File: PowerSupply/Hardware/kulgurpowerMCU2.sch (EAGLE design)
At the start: 140 parts, among them IC2 TPS77333DGK, IC3 REG1117-5, U1 MPU-6000QFN-24, U2 MPU-6000QFN-24, X1 12Mhz

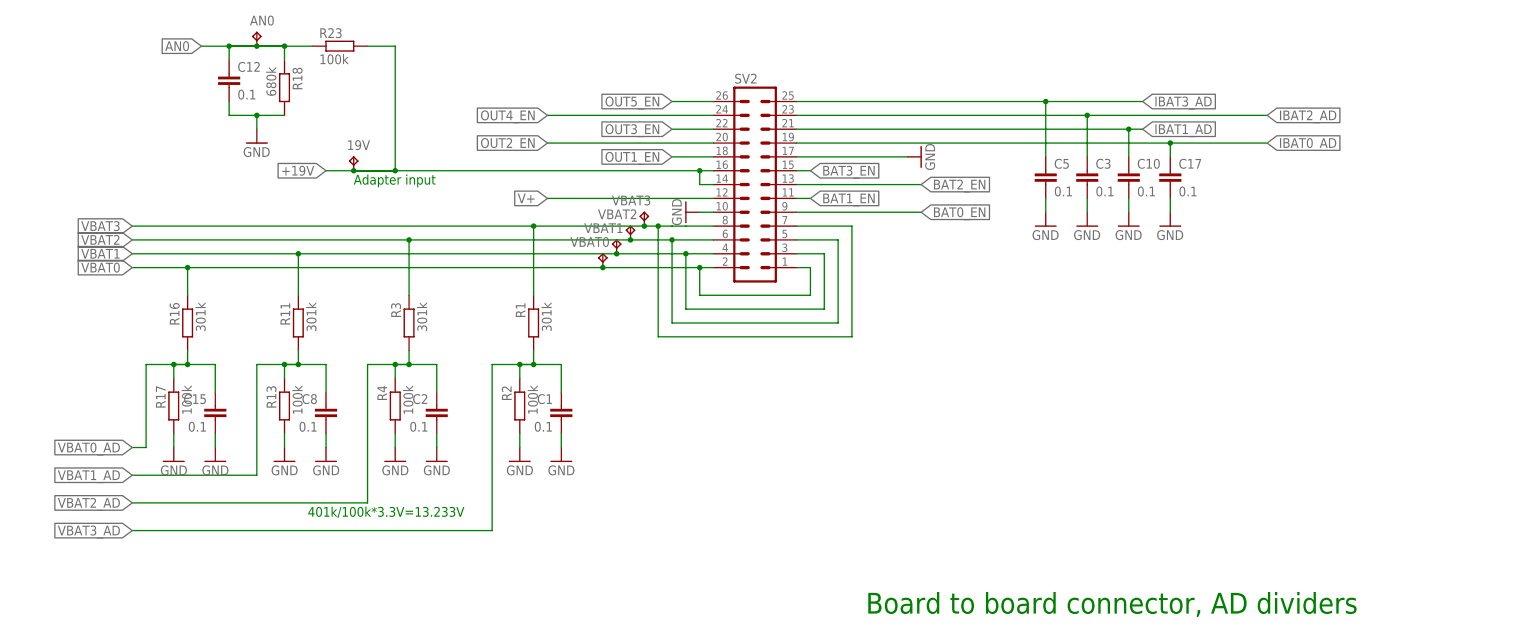
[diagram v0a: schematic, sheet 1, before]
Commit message: lot of work done on schematics
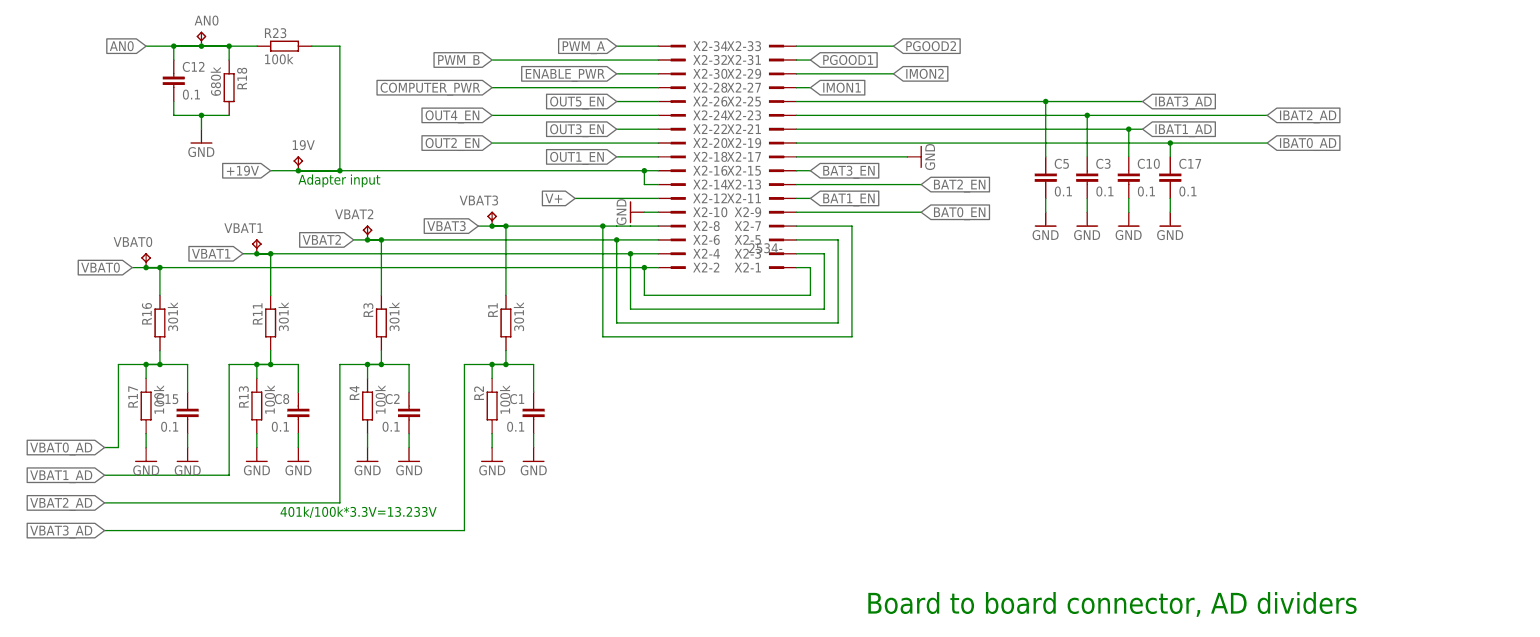
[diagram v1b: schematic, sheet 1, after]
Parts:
- removed SV2: (no value), con-lstb:MA13-2
- removed TP6, TP7: TPB1,27, testpad:TPB1,27
- added X2: 2534-, con-3m:2534-
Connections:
- removed net N$30: TP6.TP, U$14.PA7/A7/MISOA
- removed net N$31: TP7.TP, U$14.PC5/A21/!CS2!/!WAIT!/SCK8/RSPCKA
- new net COMPUTER_PWR: U$14.PC5/A21/!CS2!/!WAIT!/SCK8/RSPCKA, X2-28.KL
- new net ENABLE_PWR: U$14.PA7/A7/MISOA, X2-30.KL
- new net IMON1: X2-27.KL
- new net IMON2: X2-29.KL
- new net PGOOD1: X2-31.KL
- new net PGOOD2: X2-33.KL
- new net PWM_A: X2-34.KL
- new net PWM_B: X2-32.KL
- net +19V: now also X2-14.KL, X2-16.KL; no longer SV2.14, SV2.16
- net BAT0_EN: now also X2-9.KL; no longer SV2.9
- net BAT1_EN: now also X2-11.KL; no longer SV2.11
- net BAT2_EN: now also X2-13.KL; no longer SV2.13
- net BAT3_EN: now also X2-15.KL; no longer SV2.15
- net GND: now also X2-10.KL, X2-17.KL; no longer SV2.10, SV2.17
- net IBAT0_AD: now also X2-19.KL; no longer SV2.19
- net IBAT1_AD: now also X2-21.KL; no longer SV2.21
- net IBAT2_AD: now also X2-23.KL; no longer SV2.23
- net IBAT3_AD: now also X2-25.KL; no longer SV2.25
- net OUT1_EN: now also X2-18.KL; no longer SV2.18
- net OUT2_EN: now also X2-20.KL; no longer SV2.20
- net OUT3_EN: now also X2-22.KL; no longer SV2.22
- net OUT4_EN: now also X2-24.KL; no longer SV2.24
- net OUT5_EN: now also X2-26.KL; no longer SV2.26
- net V+: now also X2-12.KL; no longer SV2.12
- net VBAT0: now also X2-1.KL, X2-2.KL; no longer SV2.1, SV2.2
- net VBAT1: now also X2-3.KL, X2-4.KL; no longer SV2.3, SV2.4
- net VBAT2: now also X2-5.KL, X2-6.KL; no longer SV2.5, SV2.6
- net VBAT3: now also X2-7.KL, X2-8.KL; no longer SV2.7, SV2.8
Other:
- moved on the sheet: 19V, AN0, C1, C12, C15, C2, C8, R1, R11, R13, R16, R17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
